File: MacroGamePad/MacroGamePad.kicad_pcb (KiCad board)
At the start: 2 copper layers, 14 parts, among them SW1 SW_Push, SW2 SW_Push, SW3 SW_Push, SW4 SW_Push, SW5 SW_Push, SW6 RotaryEncoder_Switch, U1 MOUDLE-SEEEDUINO-XIAO

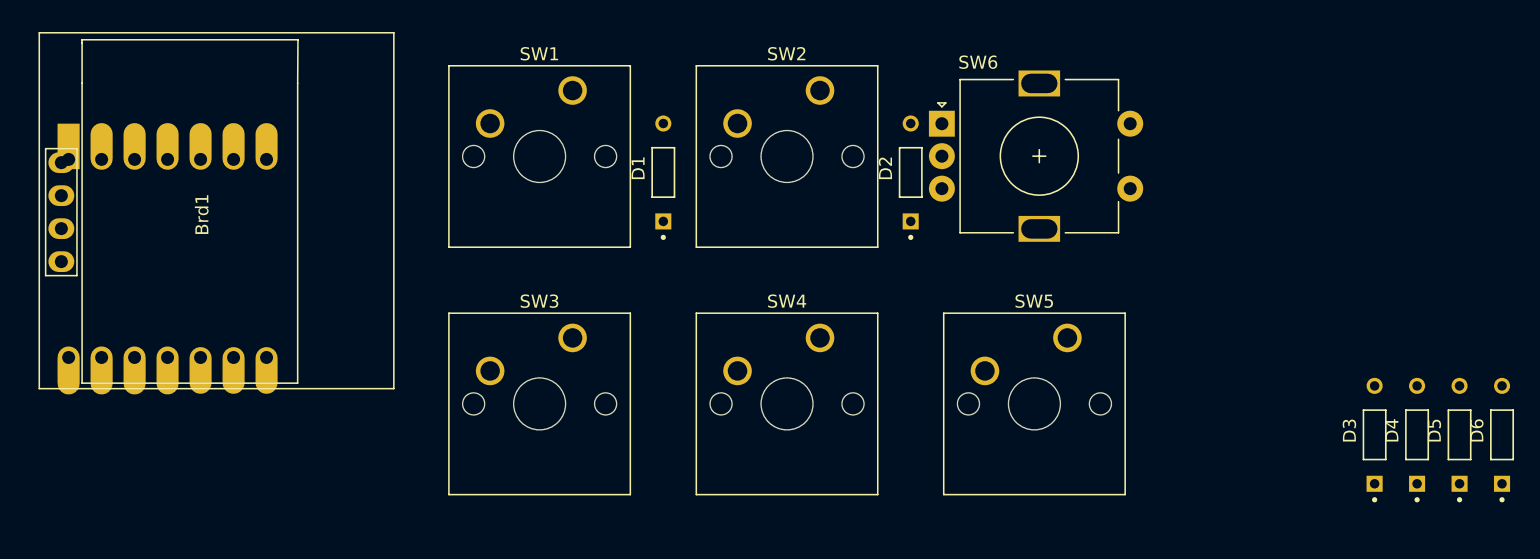
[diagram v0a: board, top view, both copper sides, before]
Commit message: PCB finished
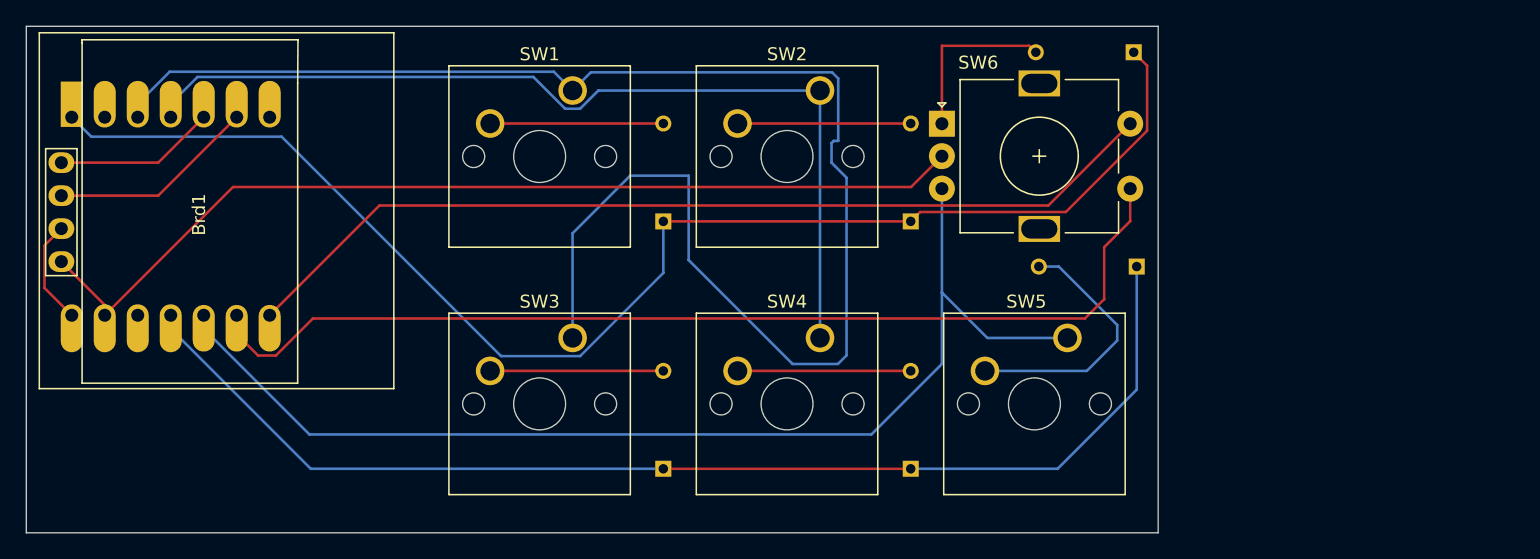
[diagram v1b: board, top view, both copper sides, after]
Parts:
- D1, D2, D3, D4, D5, D6: moved to B.Cu
- moved D3 54.8 mm to (146.0, 99.0)
- moved D6 43.6 mm to (178.5, 70.7), turned to 180 degrees
- moved D4 39.0 mm to (165.1, 99.0)
- moved D5 31.4 mm to (178.7, 87.2), turned to 180 degrees
- moved U1 3.26 mm to (108.1, 83.3)
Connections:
- U1 pad 11: unconnected-(U1-PA6_A10_D10_MOSI-Pad11) -> Row 1
- U1 pad 2: Row 1 -> unconnected-(U1-PA4_A1_D1-Pad2)
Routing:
- net Column 0: track 0.00 -> 120.7 mm
- net Row 0: track 0.00 -> 106.4 mm
- net Row 1: track 0.00 -> 91.9 mm
- net Column 2: track 0.00 -> 88.1 mm
- net RSW_S1: track 0.00 -> 80.1 mm
- net GND: track 0.00 -> 75.0 mm
- net Column 1: track 0.00 -> 72.5 mm
- net RSW_S2: track 0.00 -> 72.4 mm
- net Net-(D5-PadA): track 0.00 -> 20.3 mm
- net OLED_SCL: track 0.00 -> 16.0 mm
- net RSW_A: track 0.00 -> 13.4 mm
- net Net-(D4-PadA): track 0.00 -> 13.3 mm
- net Net-(D2-PadA): track 0.00 -> 13.3 mm
- net Net-(D3-PadA): track 0.00 -> 13.3 mm
- net Net-(D1-PadA): track 0.00 -> 13.3 mm
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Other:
- board outline added: 87.2 x 39 mm
